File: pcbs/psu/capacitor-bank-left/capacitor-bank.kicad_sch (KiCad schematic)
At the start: 25 parts, among them J1 Conn_01x03, J2 Conn_01x03

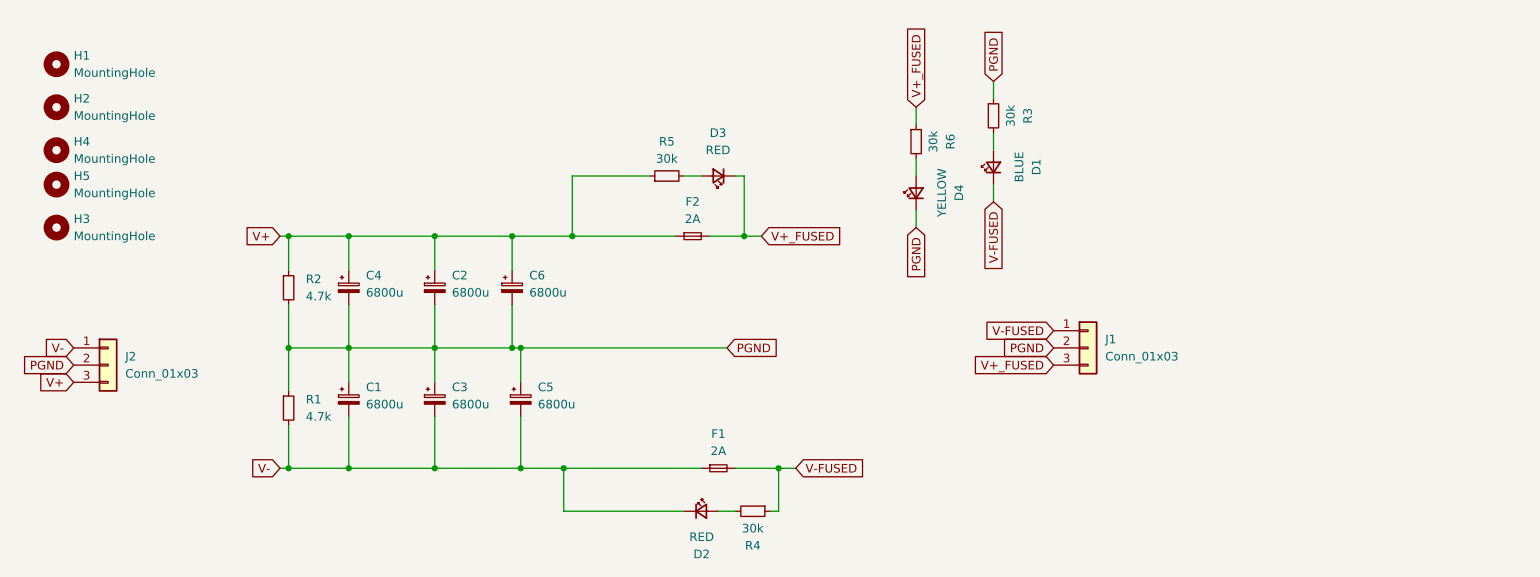
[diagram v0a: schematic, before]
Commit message: All changes
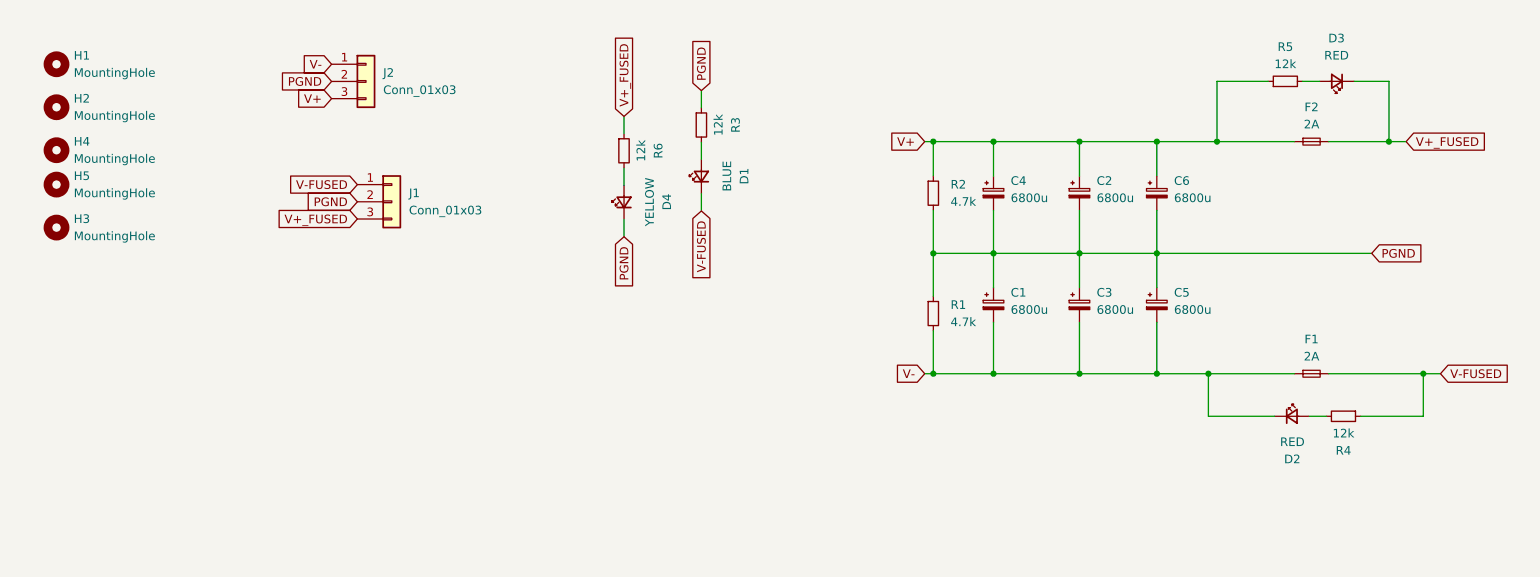
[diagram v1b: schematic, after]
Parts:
- R3, R4, R5, R6: value 30k -> 12k
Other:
- moved on the sheet: C1, C2, C3, C4, C5, C6, D1, D2, D3, D4, F1, F2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
